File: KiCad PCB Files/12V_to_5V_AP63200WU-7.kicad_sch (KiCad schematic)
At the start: 19 parts

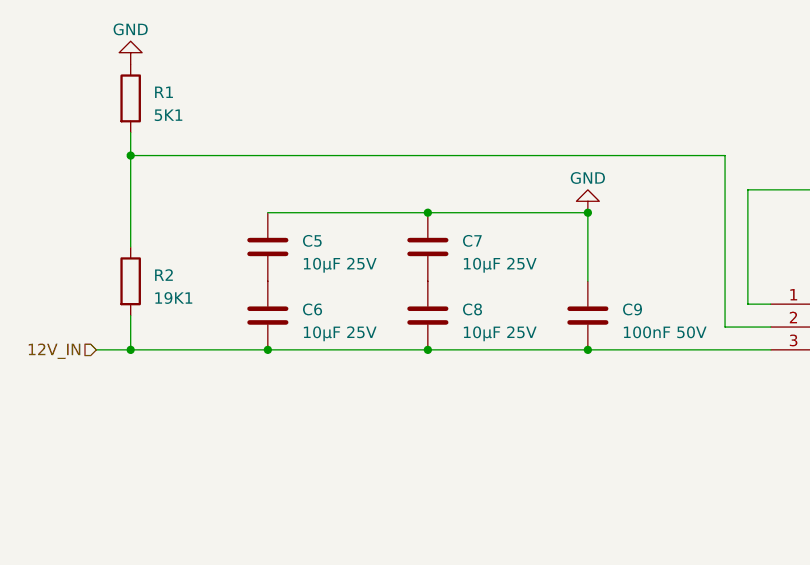
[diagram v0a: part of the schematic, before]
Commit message: Replaced input capacitors before PS1
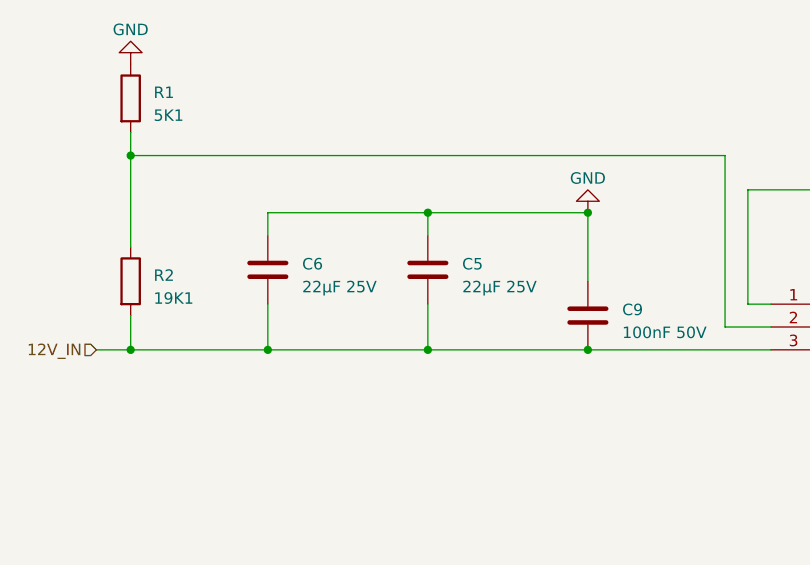
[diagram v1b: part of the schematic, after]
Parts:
- removed C7, C8: 10µF 25V, Capacitor_SMD:C_0603_1608Metric, symbol Device:C
- C5, C6: value 10µF 25V -> 22µF 25V; footprint Capacitor_SMD:C_0603_1608Metric -> Capacitor_SMD:C_1210_3225Metric; Manufacturer_Part_Number GRM188R61E106MA73J -> TMK325B7226KM-PR
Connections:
- net 12V_IN: now also C5.2
- net GND: now also C6.1
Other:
- moved on the sheet: C6
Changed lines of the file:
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@@
   (junction (at 208.28 71.12) (diameter 0) (color 0 0 0 0)
   )
+  (junction (at 191.77 71.12) (diameter 0) (color 0 0 0 0)
+  )
+  (junction (at 87.63 73.66) (diameter 0) (color 0 0 0 0)
+  )
+  (junction (at 175.26 71.12) (diameter 0) (color 0 0 0 0)
+  )
+  (junction (at 154.94 55.88) (diameter 0) (color 0 0 0 0)
+  )
+  (junction (at 36.83 52.07) (diameter 0) (color 0 0 0 0)
+  )
+  (junction (at 154.94 63.5) (diameter 0) (color 0 0 0 0)
+  )
   (junction (at 69.85 58.42) (diameter 0) (color 0 0 0 0)
   )
-  (junction (at 191.77 71.12) (diameter 0) (color 0 0 0 0)
-  )
-  (junction (at 87.63 73.66) (diameter 0) (color 0 0 0 0)
-  )
-  (junction (at 175.26 71.12) (diameter 0) (color 0 0 0 0)
-  )
-  (junction (at 154.94 55.88) (diameter 0) (color 0 0 0 0)
-  )
-  (junction (at 36.83 52.07) (diameter 0) (color 0 0 0 0)
-  )
-  (junction (at 154.94 63.5) (diameter 0) (color 0 0 0 0)
-  )
   (junction (at 224.79 71.12) (diameter 0) (color 0 0 0 0)
   )
@@
     (stroke (width 0) (type default))
   )
+  (wire (pts (xy 52.07 58.42) (xy 52.07 60.96))
+    (stroke (width 0) (type default))
+  )
   (wire (pts (xy 191.77 78.74) (xy 175.26 78.74))
     (stroke (width 0) (type default))
@@
     (stroke (width 0) (type default))
   )
+  (wire (pts (xy 69.85 58.42) (xy 87.63 58.42))
+    (stroke (width 0) (type default))
+  )
   (wire (pts (xy 105.41 55.88) (xy 142.24 55.88))
     (stroke (width 0) (type default))
@@
     (stroke (width 0) (type default))
   )
+  (wire (pts (xy 69.85 58.42) (xy 69.85 60.96))
+    (stroke (width 0) (type default))
+  )
   (wire (pts (xy 107.95 68.58) (xy 105.41 68.58))
     (stroke (width 0) (type default))
@@
     (stroke (width 0) (type default))
   )
+  (wire (pts (xy 69.85 68.58) (xy 69.85 73.66))
+    (stroke (width 0) (type default))
+  )
   (wire (pts (xy 260.35 71.12) (xy 270.51 71.12))
     (stroke (width 0) (type default))
@@
     (stroke (width 0) (type default))
   )
-  (wire (pts (xy 69.85 58.42) (xy 87.63 58.42))
-    (stroke (width 0) (type default))
-  )
   (wire (pts (xy 154.94 63.5) (xy 175.26 63.5))
     (stroke (width 0) (type default))
@@
   )
   (wire (pts (xy 242.57 71.12) (xy 252.73 71.12))
+    (stroke (width 0) (type default))
+  )
+  (wire (pts (xy 52.07 68.58) (xy 52.07 73.66))
     (stroke (width 0) (type default))
   )
@@
     )
   )
-  (symbol (lib_id "Device:C") (at 52.07 62.23 0) (unit 1)
-    (in_bom yes) (on_board yes) (dnp no) (fields_autoplaced)
-    (property "Reference" "C5" (at 55.88 61.595 0)
-      (effects (font (size 1.27 1.27)) (justify left))
-    )
-    (property "Value" "10µF 25V" (at 55.88 64.135 0)
-      (effects (font (size 1.27 1.27)) (justify left))
-    )
-    (property "Footprint" "Capacitor_SMD:C_0603_1608Metric" (at 53.0352 66.04 0)
-      (effects (font (size 1.27 1.27)) hide)
-    )
-    (property "Datasheet" "~" (at 52.07 62.23 0)
-      (effects (font (size 1.27 1.27)) hide)
-    )
-    (property "Description" "CAP CHIP 0603 10uF 25V X5R 20%" (at 52.07 62.23 0)
-      (effects (font (size 1.27 1.27)) hide)
-    )
-    (property "Manufacturer_Part_Number" "GRM188R61E106MA73J" (at 52.07 62.23 0)
-      (effects (font (size 1.27 1.27)) hide)
-    )
-    (pin "1")
-    (pin "2")
-    (instances
-      (project "VXDash"
-        (path "/f2858fc4-50de-4ff0-a01c-5b985ee14aef/e4c69d46-7a64-435d-9e3a-d73acbe7ec2b"
-          (reference "C5") (unit 1)
-        )
-      )
-    )
-  )
   (symbol (lib_id "power:GND") (at 134.62 77.47 0) (unit 1)
     (in_bom yes) (on_board yes) (dnp no) (fields_autoplaced)
@@
     )
   )
-  (symbol (lib_id "Device:C") (at 69.85 62.23 0) (unit 1)
-    (in_bom yes) (on_board yes) (dnp no) (fields_autoplaced)
-    (property "Reference" "C7" (at 73.66 61.595 0)
-      (effects (font (size 1.27 1.27)) (justify left))
-    )
-    (property "Value" "10µF 25V" (at 73.66 64.135 0)
-      (effects (font (size 1.27 1.27)) (justify left))
-    )
-    (property "Footprint" "Capacitor_SMD:C_0603_1608Metric" (at 70.8152 66.04 0)
-      (effects (font (size 1.27 1.27)) hide)
-    )
-    (property "Datasheet" "~" (at 69.85 62.23 0)
-      (effects (font (size 1.27 1.27)) hide)
-    )
-    (property "Description" "CAP CHIP 0603 10uF 25V X5R 20%" (at 69.85 62.23 0)
-      (effects (font (size 1.27 1.27)) hide)
-    )
-    (property "Manufacturer_Part_Number" "GRM188R61E106MA73J" (at 69.85 62.23 0)
-      (effects (font (size 1.27 1.27)) hide)
-    )
-    (pin "1")
-    (pin "2")
-    (instances
-      (project "VXDash"
-        (path "/f2858fc4-50de-4ff0-a01c-5b985ee14aef/e4c69d46-7a64-435d-9e3a-d73acbe7ec2b"
-          (reference "C7") (unit 1)
-        )
-      )
-    )
-  )
   (symbol (lib_id "Device:R") (at 154.94 59.69 0) (unit 1)
     (in_bom yes) (on_board yes) (dnp no) (fields_autoplaced)
@@
     )
   )
-  (symbol (lib_id "Device:C") (at 52.07 69.85 0) (unit 1)
-    (in_bom yes) (on_board yes) (dnp no) (fields_autoplaced)
-    (property "Reference" "C6" (at 55.88 69.215 0)
-      (effects (font (size 1.27 1.27)) (justify left))
-    )
-    (property "Value" "10µF 25V" (at 55.88 71.755 0)
-      (effects (font (size 1.27 1.27)) (justify left))
-    )
-    (property "Footprint" "Capacitor_SMD:C_0603_1608Metric" (at 53.0352 73.66 0)
-      (effects (font (size 1.27 1.27)) hide)
-    )
-    (property "Datasheet" "~" (at 52.07 69.85 0)
-      (effects (font (size 1.27 1.27)) hide)
-    )
-    (property "Description" "CAP CHIP 0603 10uF 25V X5R 20%" (at 52.07 69.85 0)
-      (effects (font (size 1.27 1.27)) hide)
-    )
-    (property "Manufacturer_Part_Number" "GRM188R61E106MA73J" (at 52.07 69.85 0)
+  (symbol (lib_id "Device:C") (at 52.07 64.77 0) (unit 1)
+    (in_bom yes) (on_board yes) (dnp no) (fields_autoplaced)
+    (property "Reference" "C6" (at 55.88 64.135 0)
+      (effects (font (size 1.27 1.27)) (justify left))
+    )
+    (property "Value" "22µF 25V" (at 55.88 66.675 0)
+      (effects (font (size 1.27 1.27)) (justify left))
+    )
+    (property "Footprint" "Capacitor_SMD:C_1210_3225Metric" (at 53.0352 68.58 0)
+      (effects (font (size 1.27 1.27)) hide)
+    )
+    (property "Datasheet" "~" (at 52.07 64.77 0)
+      (effects (font (size 1.27 1.27)) hide)
+    )
+    (property "Description" "CAP CER 22UF 25V X7R 1210" (at 52.07 64.77 0)
+      (effects (font (size 1.27 1.27)) hide)
+    )
+    (property "Manufacturer_Part_Number" "TMK325B7226KM-PR" (at 52.07 64.77 0)
       (effects (font (size 1.27 1.27)) hide)
     )
@@
     )
   )
-  (symbol (lib_id "Device:C") (at 69.85 69.85 0) (unit 1)
-    (in_bom yes) (on_board yes) (dnp no) (fields_autoplaced)
-    (property "Reference" "C8" (at 73.66 69.215 0)
-      (effects (font (size 1.27 1.27)) (justify left))
-    )
-    (property "Value" "10µF 25V" (at 73.66 71.755 0)
-      (effects (font (size 1.27 1.27)) (justify left))
-    )
-    (property "Footprint" "Capacitor_SMD:C_0603_1608Metric" (at 70.8152 73.66 0)
-      (effects (font (size 1.27 1.27)) hide)
-    )
-    (property "Datasheet" "~" (at 69.85 69.85 0)
-      (effects (font (size 1.27 1.27)) hide)
-    )
-    (property "Description" "CAP CHIP 0603 10uF 25V X5R 20%" (at 69.85 69.85 0)
-      (effects (font (size 1.27 1.27)) hide)
-    )
-    (property "Manufacturer_Part_Number" "GRM188R61E106MA73J" (at 69.85 69.85 0)
-      (effects (font (size 1.27 1.27)) hide)
-    )
-    (pin "1")
-    (pin "2")
-    (instances
-      (project "VXDash"
-        (path "/f2858fc4-50de-4ff0-a01c-5b985ee14aef/e4c69d46-7a64-435d-9e3a-d73acbe7ec2b"
-          (reference "C8") (unit 1)
-        )
-      )
-    )
-  )
   (symbol (lib_id "power:GND") (at 154.94 43.18 180) (unit 1)
     (in_bom yes) (on_board yes) (dnp no) (fields_autoplaced)
@@
         )
       )
+    )
+  )
+  (symbol (lib_id "Device:C") (at 69.85 64.77 0) (unit 1)
+    (in_bom yes) (on_board yes) (dnp no) (fields_autoplaced)
+    (property "Reference" "C5" (at 73.66 64.135 0)
+      (effects (font (size 1.27 1.27)) (justify left))
+    )
+    (property "Value" "22µF 25V" (at 73.66 66.675 0)
+      (effects (font (size 1.27 1.27)) (justify left))
+    )
+    (property "Footprint" "Capacitor_SMD:C_1210_3225Metric" (at 70.8152 68.58 0)
+      (effects (font (size 1.27 1.27)) hide)
+    )
+    (property "Datasheet" "~" (at 69.85 64.77 0)
+      (effects (font (size 1.27 1.27)) hide)
+    )
+    (property "Description" "CAP CER 22UF 25V X7R 1210" (at 69.85 64.77 0)
+      (effects (font (size 1.27 1.27)) hide)
+    )
+    (property "Manufacturer_Part_Number" "TMK325B7226KM-PR" (at 69.85 64.77 0)
+      (effects (font (size 1.27 1.27)) hide)
+    )
+    (pin "1")
+    (pin "2")
+    (instances
+      (project "VXDash"
+        (path "/f2858fc4-50de-4ff0-a01c-5b985ee14aef/e4c69d46-7a64-435d-9e3a-d73acbe7ec2b"
+          (reference "C5") (unit 1)
+        )
+      )
